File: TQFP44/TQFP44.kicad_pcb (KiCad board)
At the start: 2 copper layers, 56.1 x 20.6 mm, 12 parts, among them J1 Conn_01x22, J2 Conn_01x22, J3 Conn_02x22_Counter_Clockwise, J4 Conn_02x22_Counter_Clockwise, J5 Conn_02x22_Counter_Clockwise, J6 Conn_01x06

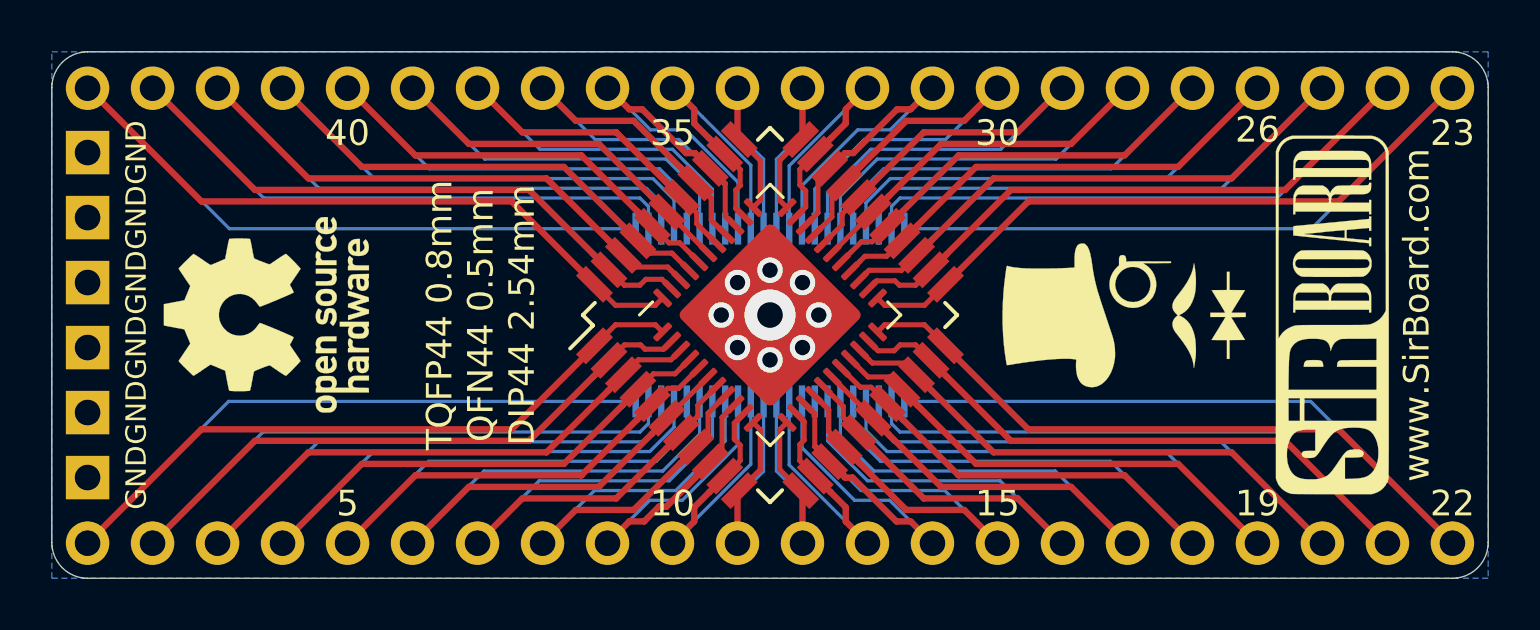
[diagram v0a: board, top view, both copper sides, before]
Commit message: Board Updates
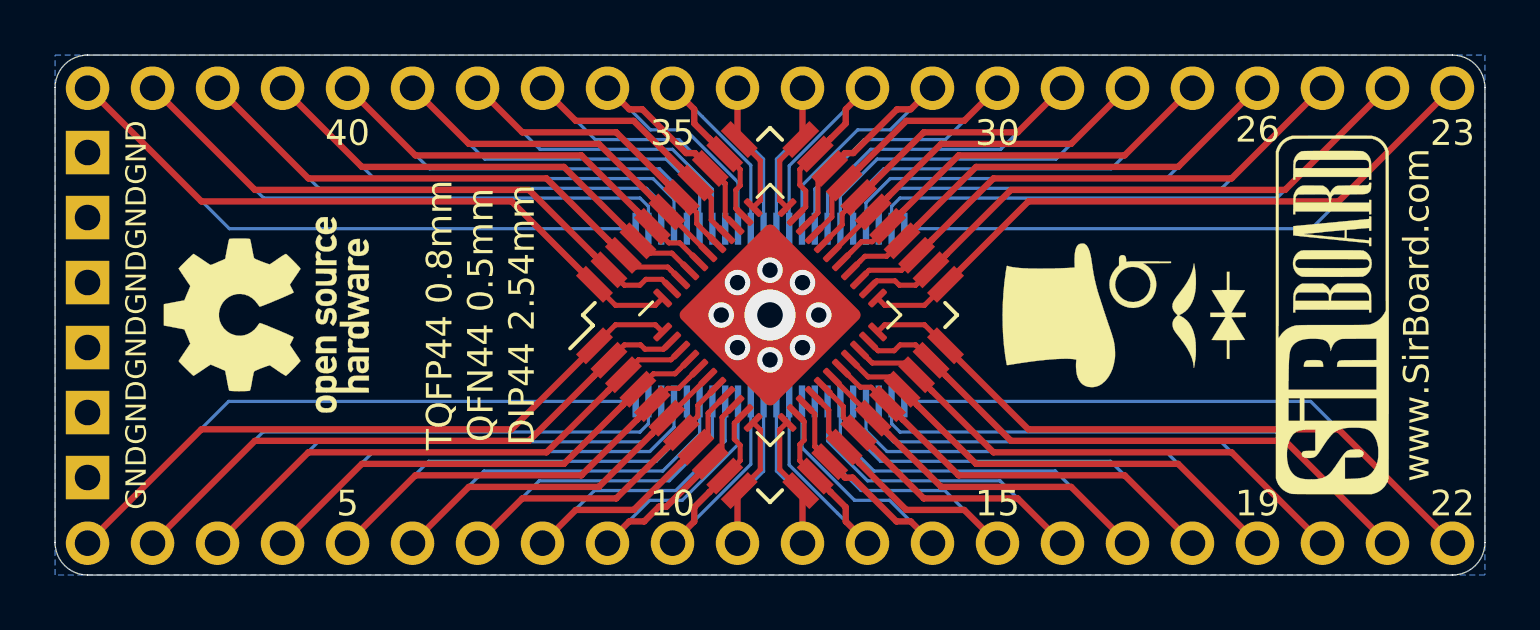
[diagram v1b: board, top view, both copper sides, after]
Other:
- board size 56.1 x 20.6 mm -> 55.9 x 20.3 mm
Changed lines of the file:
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@@
     (0 F.Cu signal)
     (31 B.Cu signal)
-    (32 B.Adhes user)
-    (33 F.Adhes user)
-    (34 B.Paste user)
-    (35 F.Paste user)
+    (32 B.Adhes user hide)
+    (33 F.Adhes user hide)
+    (34 B.Paste user hide)
+    (35 F.Paste user hide)
     (36 B.SilkS user)
     (37 F.SilkS user)
-    (38 B.Mask user)
-    (39 F.Mask user)
+    (38 B.Mask user hide)
+    (39 F.Mask user hide)
     (40 Dwgs.User user)
     (41 Cmts.User user hide)
@@
       (xy -6.38175 -2.199822) (xy 6.399893 -2.199822) (xy 6.472464 -2.17505)) (layer F.SilkS) (width 0.01))
   )
+  (gr_arc (start 94.615 43.942) (end 94.615 45.212) (angle -90) (layer Edge.Cuts) (width 0.05))
+  (gr_arc (start 41.275 43.942) (end 40.005 43.942) (angle -90) (layer Edge.Cuts) (width 0.05))
+  (gr_arc (start 41.275 26.162) (end 41.275 24.892) (angle -90) (layer Edge.Cuts) (width 0.05))
+  (gr_arc (start 94.615 26.162) (end 95.885 26.162) (angle -90) (layer Edge.Cuts) (width 0.05))
   (gr_text 44 (at 94.615 27.813) (layer B.SilkS)
     (effects (font (size 1 1) (thickness 0.15)) (justify mirror))
@@
     (effects (font (size 1 1) (thickness 0.15)) (justify mirror))
   )
-  (dimension 56.134 (width 0.15) (layer Dwgs.User)
-    (gr_text "56.134 mm" (at 67.945 18.6898) (layer Dwgs.User)
+  (dimension 55.88 (width 0.15) (layer Dwgs.User)
+    (gr_text "55.880 mm" (at 67.945 18.766) (layer Dwgs.User)
       (effects (font (size 1 1) (thickness 0.15)) hide)
     )
-    (feature1 (pts (xy 96.012 24.765) (xy 96.012 19.403379)))
-    (feature2 (pts (xy 39.878 24.765) (xy 39.878 19.403379)))
-    (crossbar (pts (xy 39.878 19.9898) (xy 96.012 19.9898)))
-    (arrow1a (pts (xy 96.012 19.9898) (xy 94.885496 20.576221)))
-    (arrow1b (pts (xy 96.012 19.9898) (xy 94.885496 19.403379)))
-    (arrow2a (pts (xy 39.878 19.9898) (xy 41.004504 20.576221)))
-    (arrow2b (pts (xy 39.878 19.9898) (xy 41.004504 19.403379)))
+    (feature1 (pts (xy 95.885 26.162) (xy 95.885 19.479579)))
+    (feature2 (pts (xy 40.005 26.162) (xy 40.005 19.479579)))
+    (crossbar (pts (xy 40.005 20.066) (xy 95.885 20.066)))
+    (arrow1a (pts (xy 95.885 20.066) (xy 94.758496 20.652421)))
+    (arrow1b (pts (xy 95.885 20.066) (xy 94.758496 19.479579)))
+    (arrow2a (pts (xy 40.005 20.066) (xy 41.131504 20.652421)))
+    (arrow2b (pts (xy 40.005 20.066) (xy 41.131504 19.479579)))
   )
-  (dimension 20.574 (width 0.15) (layer Dwgs.User)
-    (gr_text "20.574 mm" (at 33.955298 35.052 270) (layer Dwgs.User)
+  (dimension 20.32 (width 0.15) (layer Dwgs.User)
+    (gr_text "20.320 mm" (at 34.387 35.052 270) (layer Dwgs.User)
       (effects (font (size 1 1) (thickness 0.15)) hide)
     )
-    (feature1 (pts (xy 39.878 45.339) (xy 34.668877 45.339)))
-    (feature2 (pts (xy 39.878 24.765) (xy 34.668877 24.765)))
-    (crossbar (pts (xy 35.255298 24.765) (xy 35.255298 45.339)))
-    (arrow1a (pts (xy 35.255298 45.339) (xy 34.668877 44.212496)))
-    (arrow1b (pts (xy 35.255298 45.339) (xy 35.841719 44.212496)))
-    (arrow2a (pts (xy 35.255298 24.765) (xy 34.668877 25.891504)))
-    (arrow2b (pts (xy 35.255298 24.765) (xy 35.841719 25.891504)))
+    (feature1 (pts (xy 41.275 45.212) (xy 35.100579 45.212)))
+    (feature2 (pts (xy 41.275 24.892) (xy 35.100579 24.892)))
+    (crossbar (pts (xy 35.687 24.892) (xy 35.687 45.212)))
+    (arrow1a (pts (xy 35.687 45.212) (xy 35.100579 44.085496)))
+    (arrow1b (pts (xy 35.687 45.212) (xy 36.273421 44.085496)))
+    (arrow2a (pts (xy 35.687 24.892) (xy 35.100579 26.018504)))
+    (arrow2b (pts (xy 35.687 24.892) (xy 36.273421 26.018504)))
   )
   (dimension 17.78 (width 0.15) (layer Dwgs.User)
@@
     (arrow2b (pts (xy 41.275 22.6822) (xy 42.401504 22.095779)))
   )
-  (gr_arc (start 41.275 43.942) (end 39.878 43.942) (angle -90) (layer Edge.Cuts) (width 0.05))
-  (gr_arc (start 94.615 43.942) (end 94.615 45.339) (angle -90) (layer Edge.Cuts) (width 0.05))
-  (gr_arc (start 94.615 26.162) (end 96.012 26.162) (angle -90) (layer Edge.Cuts) (width 0.05))
-  (gr_arc (start 41.275 26.162) (end 41.275 24.765) (angle -90) (layer Edge.Cuts) (width 0.05))
   (gr_circle (center 67.944577 35.052) (end 68.6816 35.052) (layer B.Mask) (width 0.5))
   (gr_circle (center 67.944577 35.052) (end 68.6816 35.052) (layer F.Mask) (width 0.5))
@@
     (effects (font (size 1 1) (thickness 0.15)))
   )
-  (gr_line (start 96.012 43.942) (end 96.012 26.162) (layer Edge.Cuts) (width 0.05))
-  (gr_line (start 41.275 45.339) (end 94.615 45.339) (layer Edge.Cuts) (width 0.05))
-  (gr_line (start 39.878 26.162) (end 39.878 43.942) (layer Edge.Cuts) (width 0.05))
-  (gr_line (start 94.615 24.765) (end 41.275 24.765) (layer Edge.Cuts) (width 0.05))
+  (gr_line (start 95.885 43.942) (end 95.885 26.162) (layer Edge.Cuts) (width 0.05))
+  (gr_line (start 41.275 45.212) (end 94.615 45.212) (layer Edge.Cuts) (width 0.05))
+  (gr_line (start 40.005 26.162) (end 40.005 43.942) (layer Edge.Cuts) (width 0.05))
+  (gr_line (start 94.615 24.892) (end 41.275 24.892) (layer Edge.Cuts) (width 0.05))
   (segment (start 72.143447 34.389087) (end 72.42536 34.671) (width 0.2) (layer F.Cu) (net 1))
   (segment (start 73.982854 34.671) (end 74.803936 33.849918) (width 0.2) (layer F.Cu) (net 1))
@@
     (polygon
       (pts
-        (xy 39.878 24.765) (xy 96.012 24.765) (xy 96.012 45.339) (xy 39.878 45.339)
+        (xy 40.005 24.892) (xy 95.885 24.892) (xy 95.885 45.212) (xy 40.005 45.212)
       )
     )
